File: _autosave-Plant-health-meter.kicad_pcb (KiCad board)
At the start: 4 copper layers, 121.2 x 25 mm, 75 parts, among them J1 Conn_01x02, J2 Conn_01x02, J3 Conn_01x04, J4 UJ2-MIBH2-4-SMT-TR, J5 Conn_01x02, Q1 AO3401A, SW1 Boot, SW2 Reset, U1 LTC4412xS6, U2 TPS62172DSG, U3 USBLC6-2P6, U4 ESP32-C3FH4X, U5 BME280, U7 TLC555xPS, Y1 40MHz

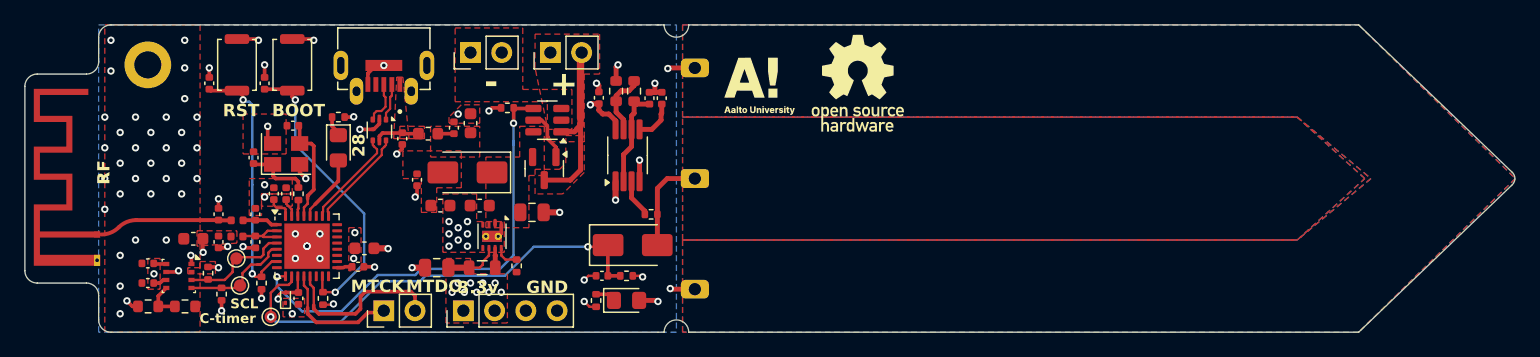
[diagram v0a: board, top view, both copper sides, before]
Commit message: Some updates
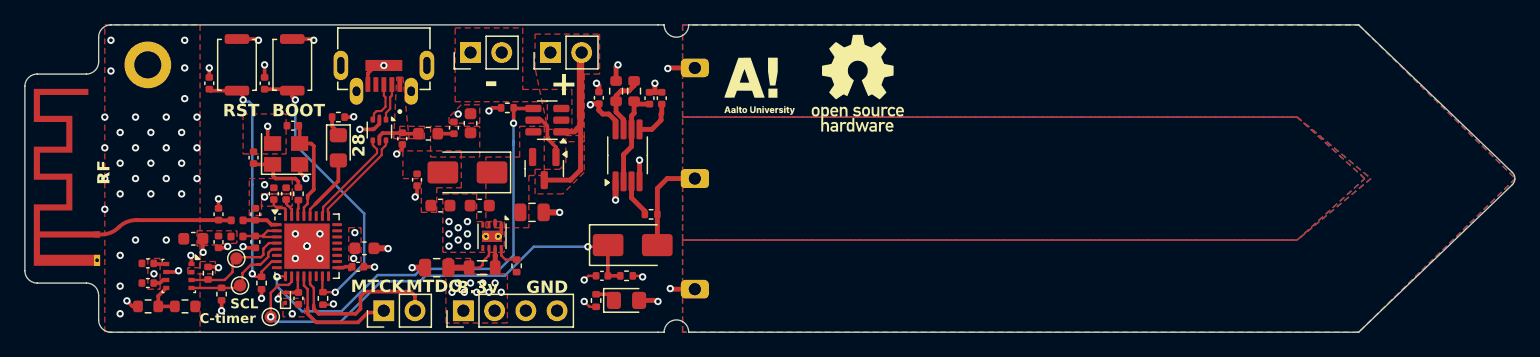
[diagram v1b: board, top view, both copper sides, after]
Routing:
- added copper zone on In2.Cu, net +3.3V
- removed copper zone on B.Cu, net +3.3V
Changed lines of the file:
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@@
 		(net 5)
 		(net_name "+3.3V")
-		(layer "B.Cu")
+		(layer "In2.Cu")
 		(hatch edge 0.5)
 		(priority 14)
